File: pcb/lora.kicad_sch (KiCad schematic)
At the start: 24 parts, among them U6 ECS-TXO-20CSMV4-320-AY-TR, U7 SX1262IMLTRT, U8 BGS12WN6E6327

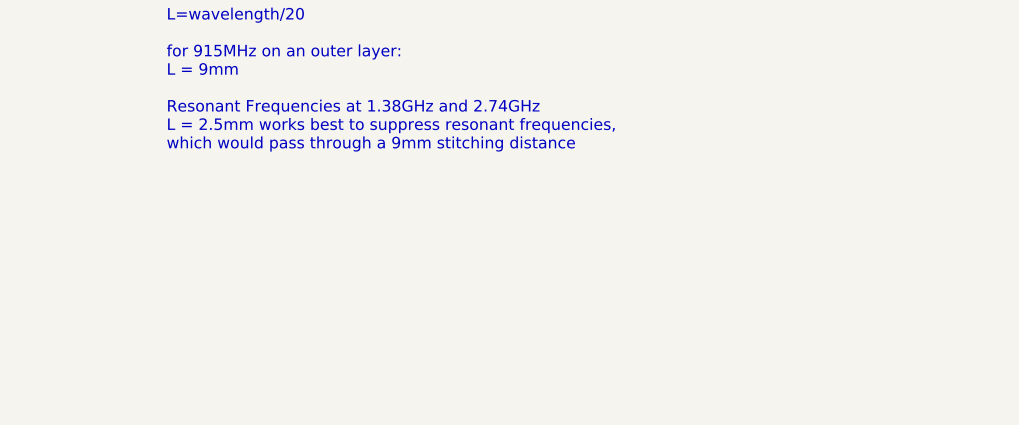
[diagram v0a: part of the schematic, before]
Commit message: V2 fixup
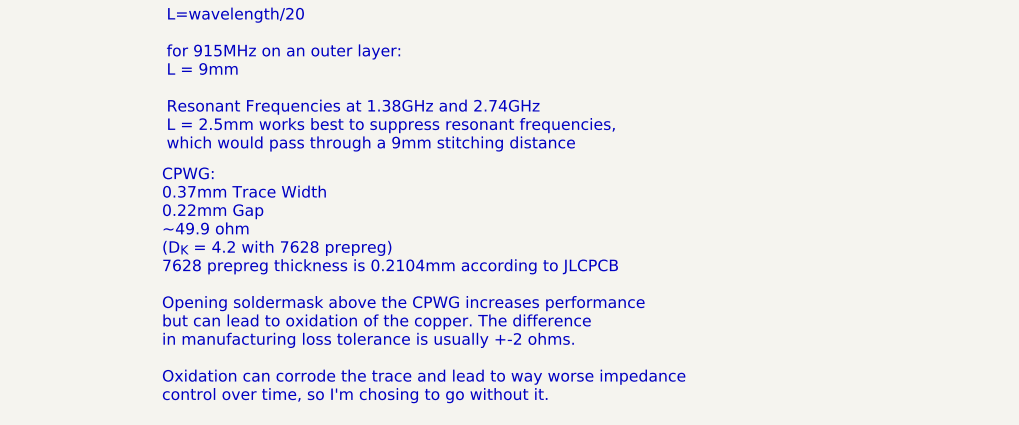
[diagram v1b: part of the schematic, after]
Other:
- note added: "CPWG: 0.37mm Trace Width 0.22mm Gap ~49.9 ohm (D_{K} = 4.2 with 7628 prepreg) 7628 prepreg thickness is 0.2104mm according to JLCPCB Opening soldermask above the CPWG increases performance but can lead to oxidation of the copper. The difference in manufacturing loss tolerance is usually +-2 ohms. Oxidation can corrode the trace and lead to way worse impedance control over time, so I'm chosing to 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"
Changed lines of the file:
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@@
 		(title "915MHz LoRa Modem")
 		(date "2026-10-09")
-		(rev "1")
+		(rev "2")
 		(company "Dylan DiBeneditto")
 	)
@@
 		)
 	)
+	(text "CPWG:\n0.37mm Trace Width\n0.22mm Gap\n~49.9 ohm\n(D_{K} = 4.2 with 7628 prepreg)\n7628 prepreg thickness is 0.2104mm according to JLCPCB\n\nOpening soldermask above the CPWG increases performance\nbut can lead to oxidation of the copper. The difference \nin manufacturing loss tolerance is usually +-2 ohms.\n\nOxidation can corrode the trace and lead to way worse impedance\ncontrol over time, so I'm chosing to go without it."
+		(exclude_from_sim no)
+		(at 92.456 180.848 0)
+		(effects
+			(font
+				(size 1.27 1.27)
+			)
+			(justify left)
+		)
+	)

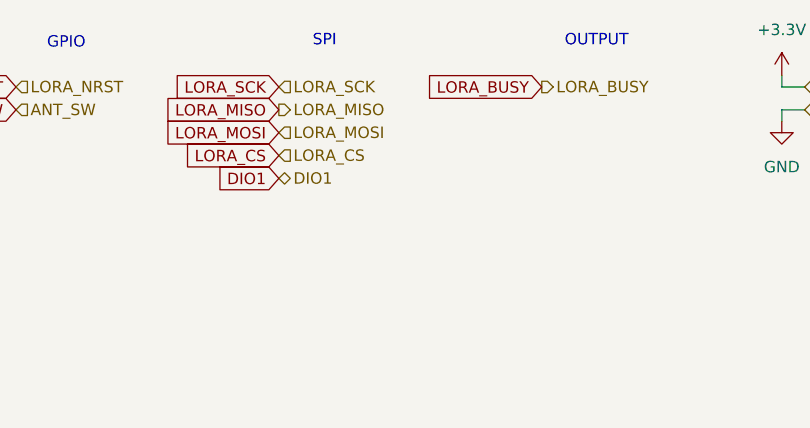
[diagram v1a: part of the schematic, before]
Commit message: revision 3
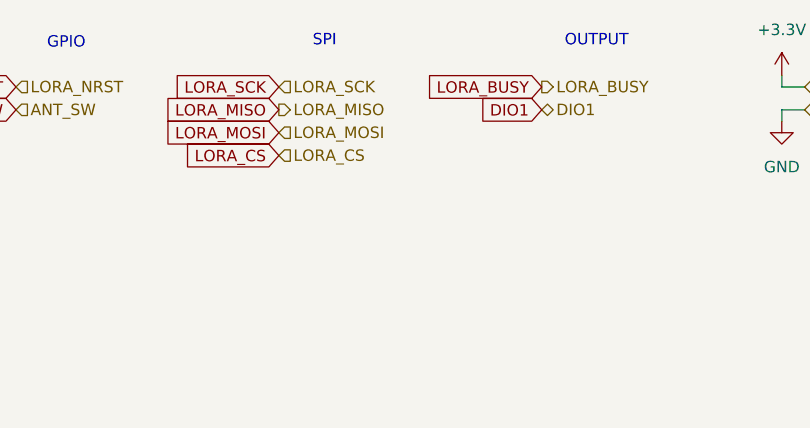
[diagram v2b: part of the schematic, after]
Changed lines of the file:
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@@
 		(title "915MHz LoRa Modem")
 		(date "2026-10-09")
-		(rev "2")
+		(rev "3")
 		(company "Dylan DiBeneditto")
 	)
@@
 	(global_label "DIO1"
 		(shape input)
-		(at 199.39 35.56 180)
+		(at 228.6 27.94 180)
 		(fields_autoplaced yes)
 		(effects
@@
 		)
 		(property "Intersheetrefs" "${INTERSHEET_REFS}"
-			(at 191.99 35.56 0)
+			(at 221.2 27.94 0)
 			(hide yes)
 			(show_name no)
@@
 	(hierarchical_label "DIO1"
 		(shape bidirectional)
-		(at 199.39 35.56 0)
-		(effects
-			(font
+		(at 228.6 27.94 0)
+		(effects
+			(font
